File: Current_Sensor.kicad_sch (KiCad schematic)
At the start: 3 parts

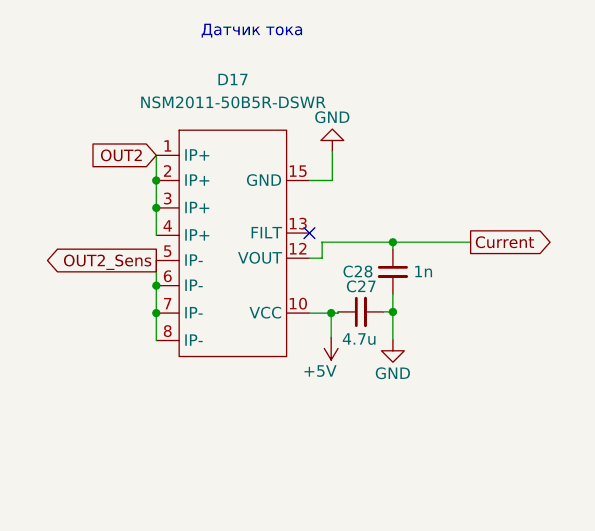
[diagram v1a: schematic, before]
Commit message: Развел все дорожки
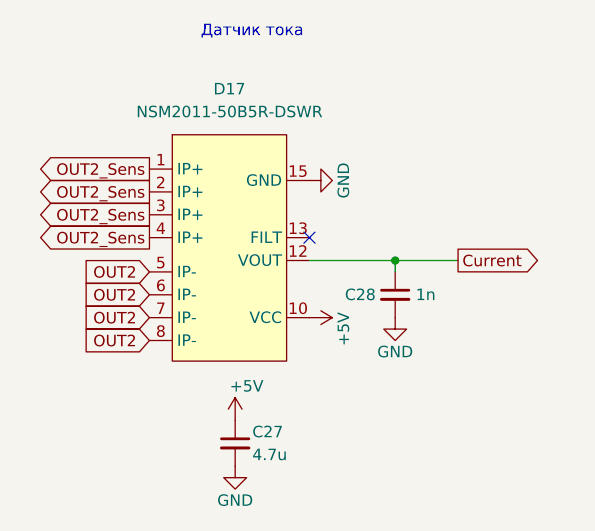
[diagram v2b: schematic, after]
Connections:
- net OUT2: now also D17.5 (IP-), D17.6 (IP-), D17.7 (IP-), D17.8 (IP-); no longer D17.1 (IP+), D17.2 (IP+), D17.3 (IP+), D17.4 (IP+)
- net OUT2_Sens: now also D17.1 (IP+), D17.2 (IP+), D17.3 (IP+), D17.4 (IP+); no longer D17.5 (IP-), D17.6 (IP-), D17.7 (IP-), D17.8 (IP-)
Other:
- moved on the sheet: C27, C28
